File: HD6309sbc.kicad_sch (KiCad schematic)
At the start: 20 parts, among them J1 Conn_01x02_Male, J3 Conn_01x02_Male, U1 HD63C09, U11 74HC02, U12 74HC21, U13 74HC21, U4 UM61256FK, U5 UM61256FK, U6 27C256, U7 74HC04, U8 74HC00

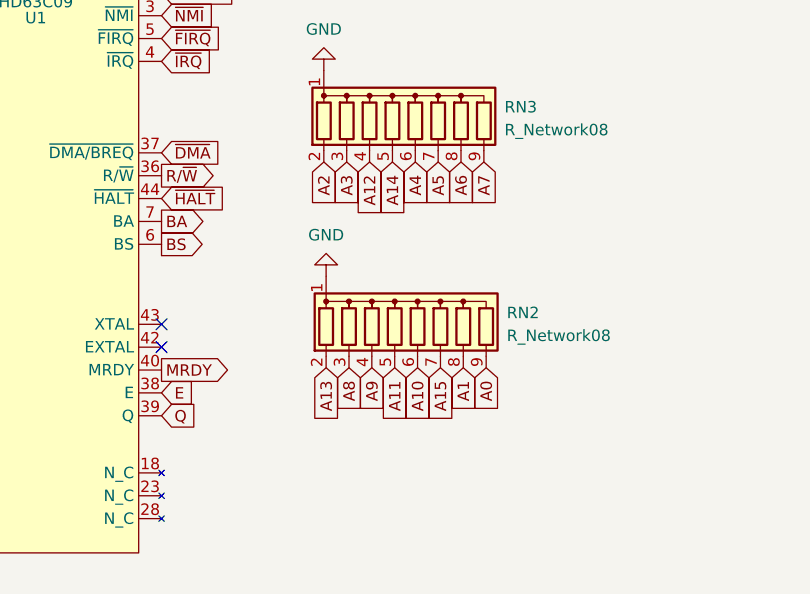
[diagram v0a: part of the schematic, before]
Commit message: rearrange components for routing
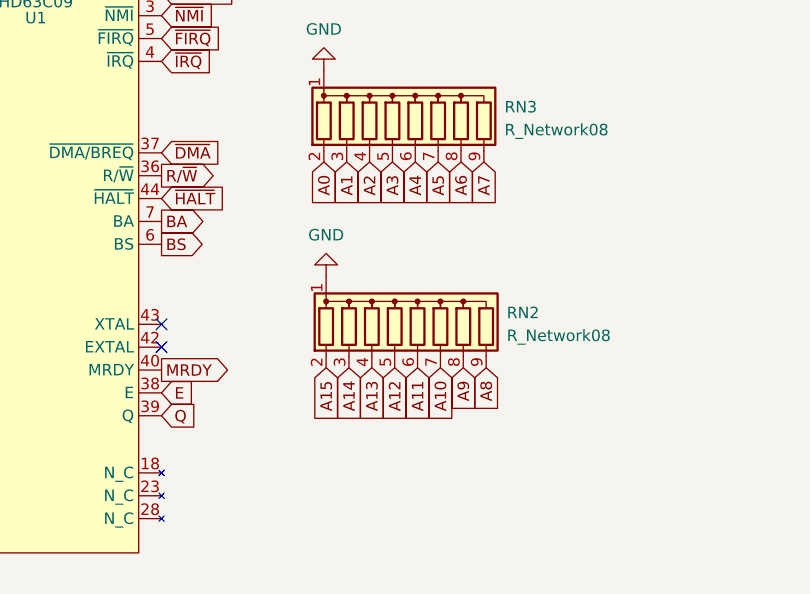
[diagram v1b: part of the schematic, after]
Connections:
- net A0: now also RN3.2 (R1); no longer RN2.9 (R8)
- net A1: now also RN3.3 (R2); no longer RN2.8 (R7)
- net A10: now also RN2.7 (R6); no longer RN2.6 (R5)
- net A11: now also RN2.6 (R5); no longer RN2.5 (R4)
- net A12: now also RN2.5 (R4); no longer RN3.4 (R3)
- net A13: now also RN2.4 (R3); no longer RN2.2 (R1)
- net A14: now also RN2.3 (R2); no longer RN3.5 (R4)
- net A15: now also RN2.2 (R1); no longer RN2.7 (R6)
- net A2: now also RN3.4 (R3); no longer RN3.2 (R1)
- net A3: now also RN3.5 (R4); no longer RN3.3 (R2)
- net A8: now also RN2.9 (R8); no longer RN2.3 (R2)
- net A9: now also RN2.8 (R7); no longer RN2.4 (R3)
